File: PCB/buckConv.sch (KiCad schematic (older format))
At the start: 12 parts, among them Q3 STL6N3LLH6, U5 LTC4440-5

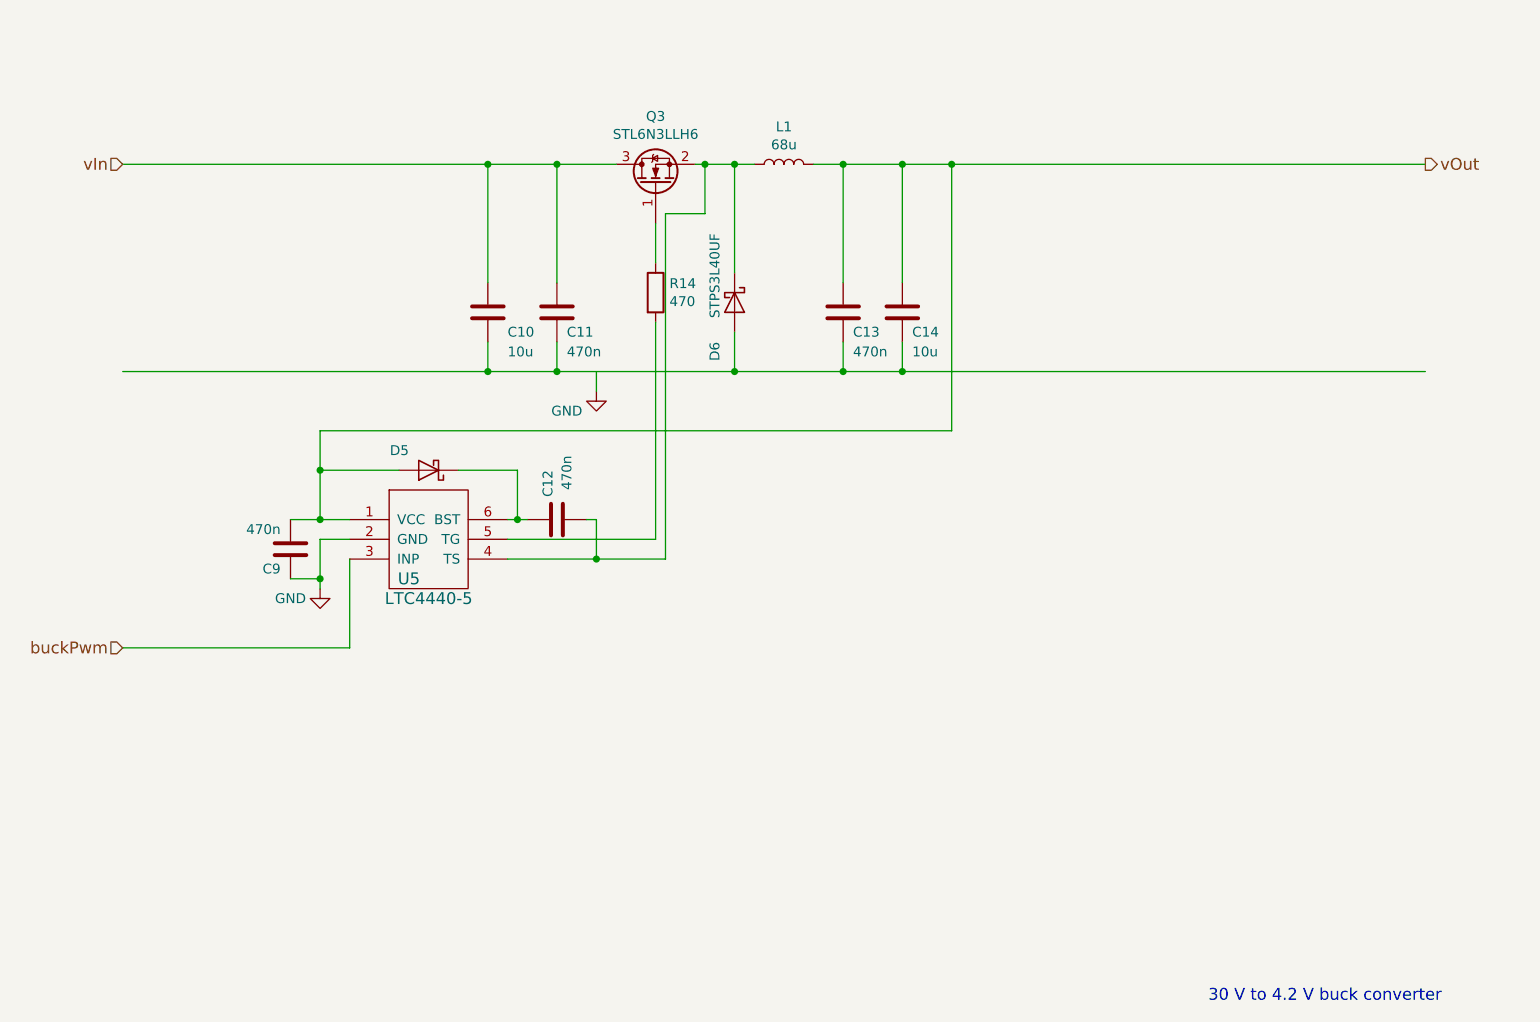
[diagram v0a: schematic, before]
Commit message: Added SEPIC ltspice model
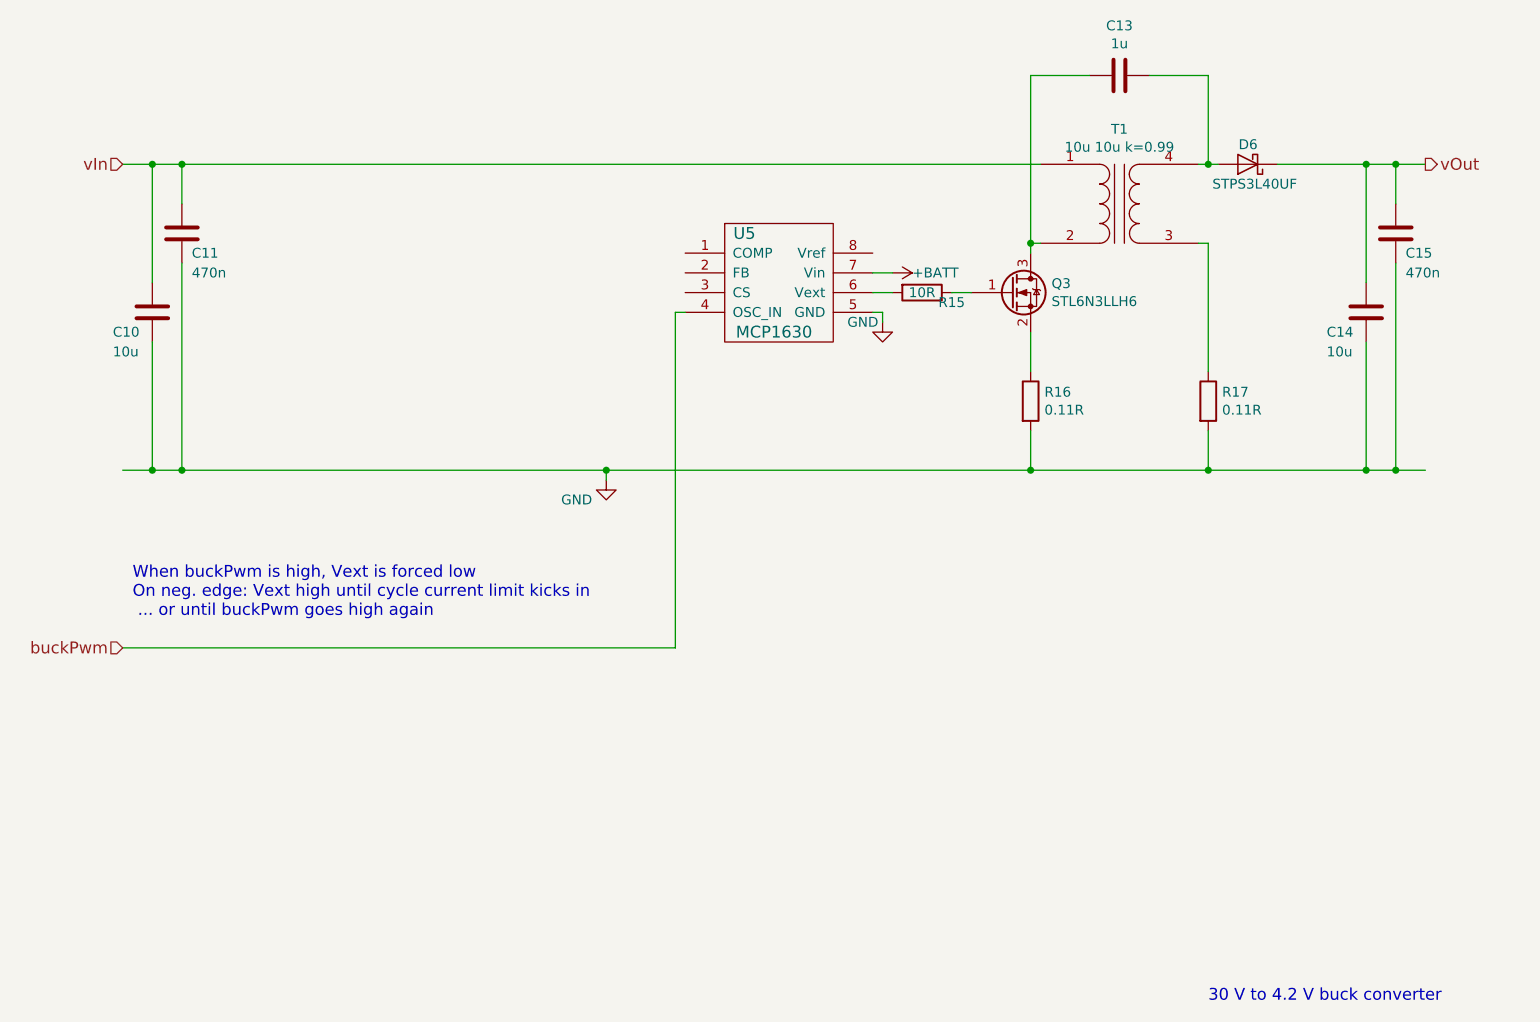
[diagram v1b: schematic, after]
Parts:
- removed C12, C9: 470n, Capacitors_SMD:C_0805, symbol C
- removed D5: B5819WS, Diodes_SMD:D_SOD-323, symbol D_Schottky
- removed L1: 68u, myStuff:MSS1048, symbol L
- removed R14: 470, Resistors_SMD:R_0805, symbol R
- removed U5: LTC4440-5, TO_SOT_Packages_SMD:SOT-23-6_Handsoldering, symbol LTC4440
- added C15: 470n, Capacitors_SMD:C_0805, symbol C
- added R15: 10R, Resistors_SMD:R_0805_HandSoldering, symbol R
- added R16, R17: 0.11R, symbol R
- added T1: 10u 10u k=0.99, symbol Transformer_1P_1S
- added U5: MCP1630, Housings_SSOP:MSOP-8_3x3mm_Pitch0.65mm, symbol MCP1630
- C13: value 470n -> 1u; footprint Capacitors_SMD:C_0805 -> (none)
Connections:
- net labels added: +BATT
- wire segments 37 -> 31
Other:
- note added: "When buckPwm is high, Vext is forced low\nOn neg. edge: Vext high until cycle current limit kicks in\n ... or until buckPwm goes high again"
- moved on the sheet: C10, C11, D6
